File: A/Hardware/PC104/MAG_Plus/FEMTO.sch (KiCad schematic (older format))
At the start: 10 parts, among them J6 Conn_01x12_Male, U11 ISO7341C

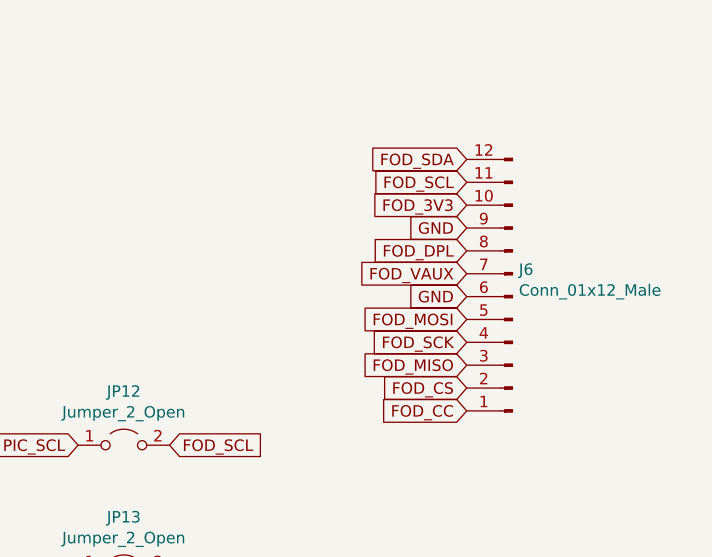
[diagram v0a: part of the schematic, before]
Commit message: PCB update
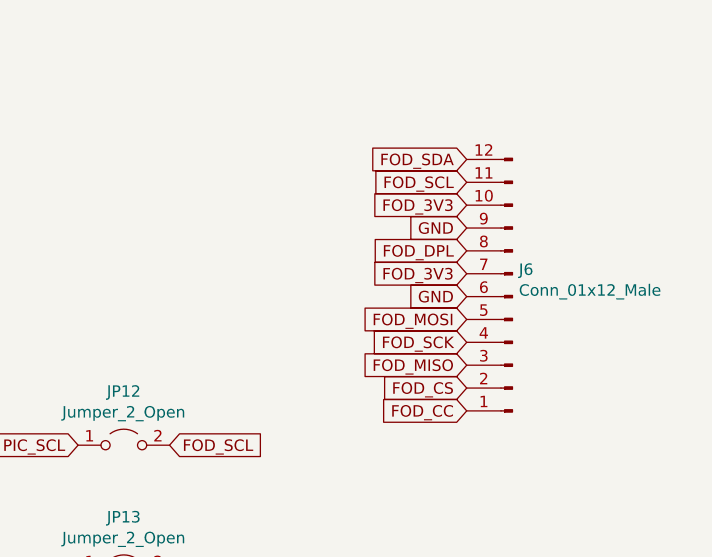
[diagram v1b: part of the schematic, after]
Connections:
- net FOD_VAUX is gone; now on net FOD_3V3: J6.7 (Pin_7)
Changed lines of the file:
@@
 GND
 Text GLabel 10300 2450 0    50   Input ~ 0
-FOD_VAUX
+FOD_3V3
 Text GLabel 10300 2350 0    50   Input ~ 0
 FOD_DPL
